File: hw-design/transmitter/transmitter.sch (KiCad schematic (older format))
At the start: 33 parts, among them P1 CONN_01X03, Q1 2N3904, Q2 2N3904, SW1 power, U1 usb-micro, U2 MCP73833, U3 CD4047, U4 CD4047

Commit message: Revision 2
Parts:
- removed D1: LED, w_indicators:led_3mm_yellow, symbol LED
- removed D3: LED, w_indicators:led_3mm_red, symbol LED
- removed RV3: 2R, Potentiometers:Potentiometer_Bourns_3296W_3-8Zoll_Inline_ScrewUp, symbol POT
- added D1: Led_x2-CA, iwasz:led_3mm-3pins, symbol Led_x2-CA
- added P10, P11, P2, P3, P4, P7: test-double, iwasz:testpad-2p, symbol test-double
- added P12: OptionC, w_pin_strip:pin_socket_2, symbol CONN_01X02
- added P5: test-double, iwasz:testpad-2p, symbol test-double-RESCUE-transmitter
- added P6: CONN_01X02, w_pin_strip:pin_socket_2, symbol CONN_01X02
- added P8: OptionB, w_pin_strip:pin_socket_2, symbol CONN_01X02
- added P9: OptionA, w_pin_strip:pin_socket_2, symbol CONN_01X02
- added R9: current sense 1R, resistor:0207%2f10, symbol R
- C1, C7: footprint w_smd_cap:c_tant_A -> iwasz:c_tant_B-pins21
- D2: value LED -> VISHAY TSAL6200; footprint w_indicators:led_3mm_green -> LEDs:LED-5MM
- D5, D6: value D -> 1N4148; footprint ref-packages-longpad:SOD80 -> ref-packages:SOD323
- P1: footprint w_conn_df13:df13-3p-125dsa -> w_pin_strip:pin_socket_3
- Q1, Q2: symbol Q_NPN_EBC -> Q_NPN_CBE
- R1: value 730R -> 20R; footprint w_smd_resistors:r_0603 -> w_smd_resistors:r_1210
- R2, R3: value 730R -> 560R
- R8: value 1k -> 2R
- RV1, RV2: footprint Potentiometers:Potentiometer_Bourns_3296W_3-8Zoll_Inline_ScrewUp -> Potentiometers:Potentiometer_Bourns_3006P_Angular_ScrewFront
- U3, U4: footprint w_smd_dil:soic-14 -> Housings_SOIC:SOIC-14_3.9x8.7mm_Pitch1.27mm
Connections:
- wire segments 111 -> 123
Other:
- note added: "300mA, 2kR = 500mA"
- note removed: "300mA"
- moved on the sheet: C2, C3, C4, C5, C6, R2, R3, R5, R8, U3, U4

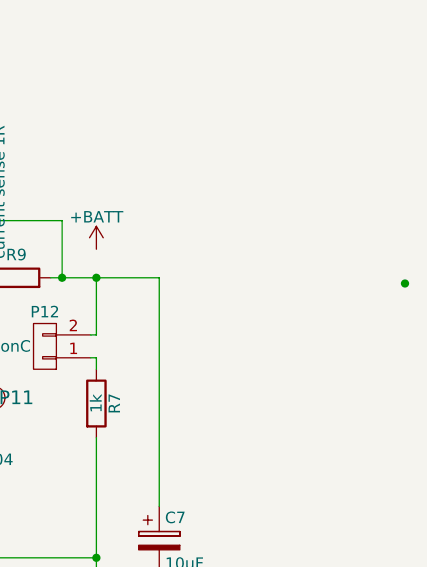
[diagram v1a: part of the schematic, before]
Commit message: Rewizja 2
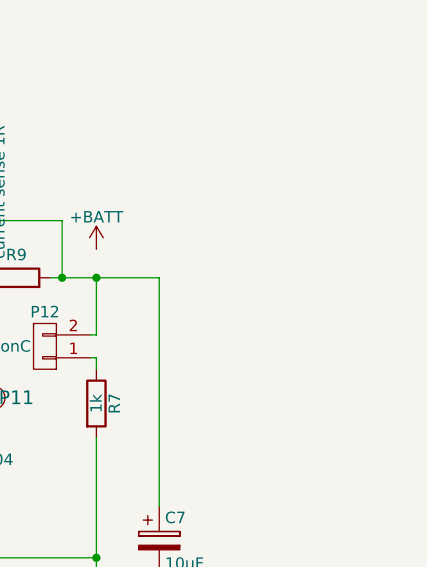
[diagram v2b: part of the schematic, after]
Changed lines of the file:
@@
 Connection ~ 2050 3950
 Connection ~ 9650 3725
-Connection ~ 11725 3225
 Wire Wire Line
 	4400 1325 4750 1325

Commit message: Funkcjonaloność tego zegara na LEDac jest w tym momencie powtórzona na LCDku
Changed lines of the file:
@@
 $EndComp
 Wire Wire Line
-	10350 3450 10375 3450
+	10375 3450 10350 3450
 Wire Wire Line
-	10375 3450 10375 3200
+	10375 3075 10375 3450
 Wire Wire Line
 	10350 3550 10375 3550

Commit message: HW changes, removed BLE, and changed chanrging and ldo circuits
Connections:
- wire segments 123 -> 125
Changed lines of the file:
@@
 	1975 3175 1975 3750
 Wire Wire Line
-	1975 3575 2050 3575
+	1975 3575 2150 3575
 Wire Wire Line
 	1975 3750 2625 3750
@@
 	4850 3175 5475 3175
 Wire Wire Line
-	5225 3575 5375 3575
+	5225 3575 5475 3575
 Wire Wire Line
 	4850 3750 5950 3750
@@
 Wire Wire Line
 	5050 1325 5050 1375
+Wire Wire Line
+	5775 3575 5875 3575
+Wire Wire Line
+	2450 3575 2550 3575
 $EndSCHEMATC
